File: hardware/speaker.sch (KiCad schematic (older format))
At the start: 9 parts, among them U11 OPA344

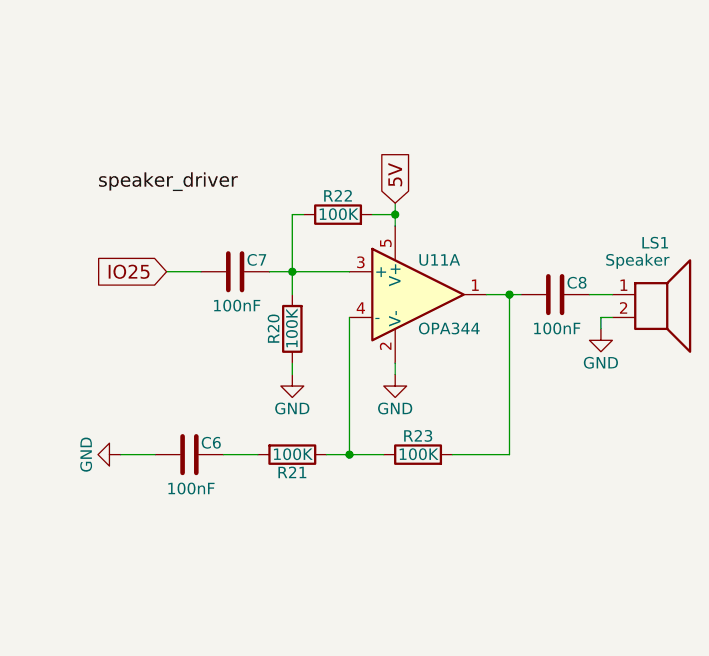
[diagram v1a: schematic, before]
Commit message: updatge
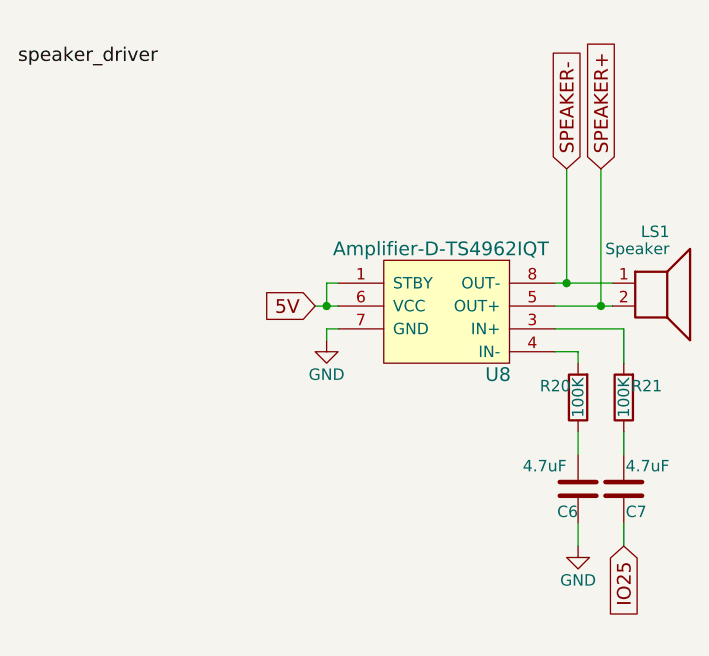
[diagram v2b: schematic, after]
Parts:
- removed C8: 100nF, Capacitors_SMD:C_0603_HandSoldering, symbol C
- removed R22, R23: 100K, Resistors_SMD:R_0603_HandSoldering, symbol R
- removed U11: OPA344, TO_SOT_Packages_SMD:SOT-23-5, symbol OPA344
- added U8: Amplifier-D-TS4962IQT, Housings_DFN_QFN:DFN-8-1EP_3x3mm_Pitch0.65mm, symbol Amplifier-D-TS4962IQT
- C6, C7: value 100nF -> 4.7uF; Part Number GRM188R71C104KA01D -> CL10B475KQ8NQNC
- R20, R21: Part Number RC0603JR-07100KL -> RC0603JR-07150KL
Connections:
- net 5V: now also U8.1 (STBY), U8.6 (VCC)
- net GND: now also C6.1, U8.7 (GND); no longer C6.2, LS1.2, R20.1
- net IO25: now also C7.1; no longer C7.2
- net at R21.1: now also C7.2
- net at R20.2: now also U8.4 (IN-); no longer C7.1
- net SPEAKER-: now reaches LS1.1
- net SPEAKER-: now also U8.8 (OUT-)
- net at R21.2: now also U8.3 (IN+); no longer C6.1
- new net: C6.2, R20.1
- new net SPEAKER+: LS1.2, U8.5 (OUT+)
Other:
- moved on the sheet: LS1
